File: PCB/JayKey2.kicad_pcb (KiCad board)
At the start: 4 copper layers, 1 part, among them U1 ATXMEGA128A1U-AU

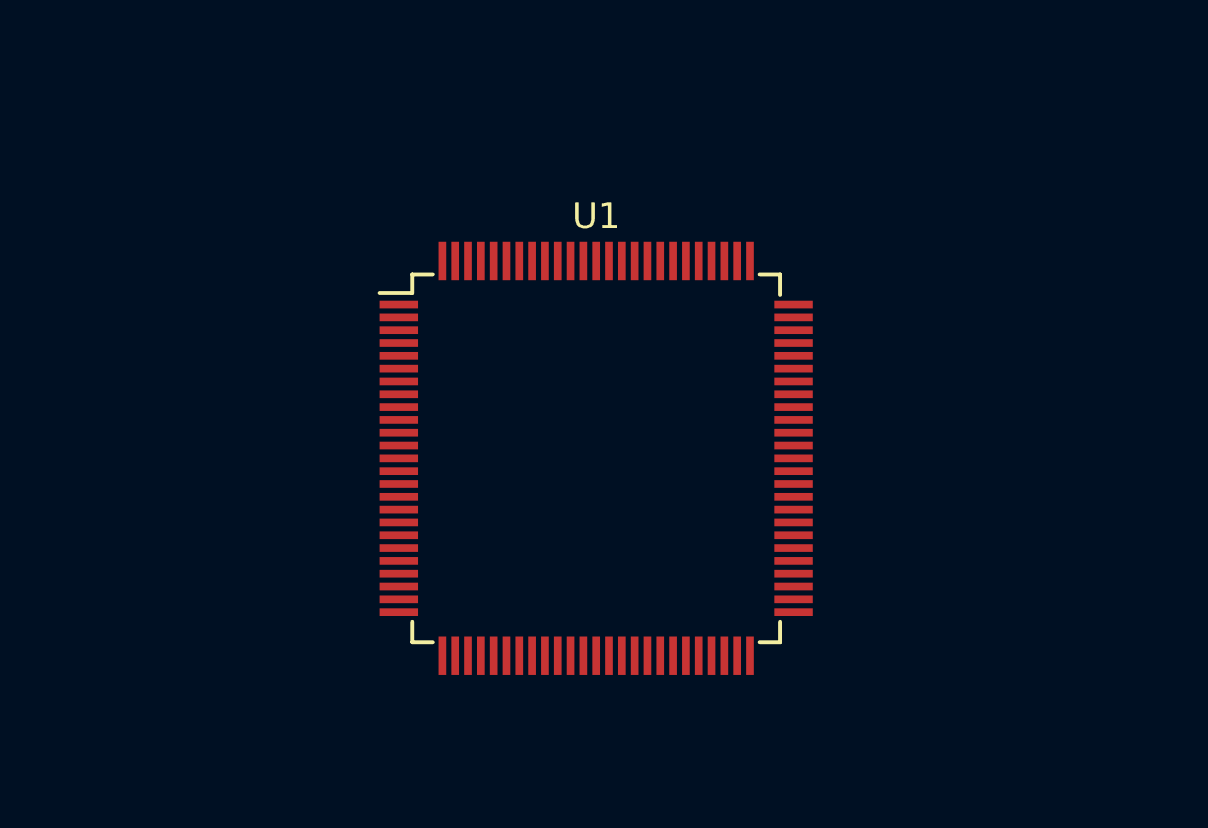
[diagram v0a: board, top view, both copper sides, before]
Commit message: 2018.03.29 Nightly
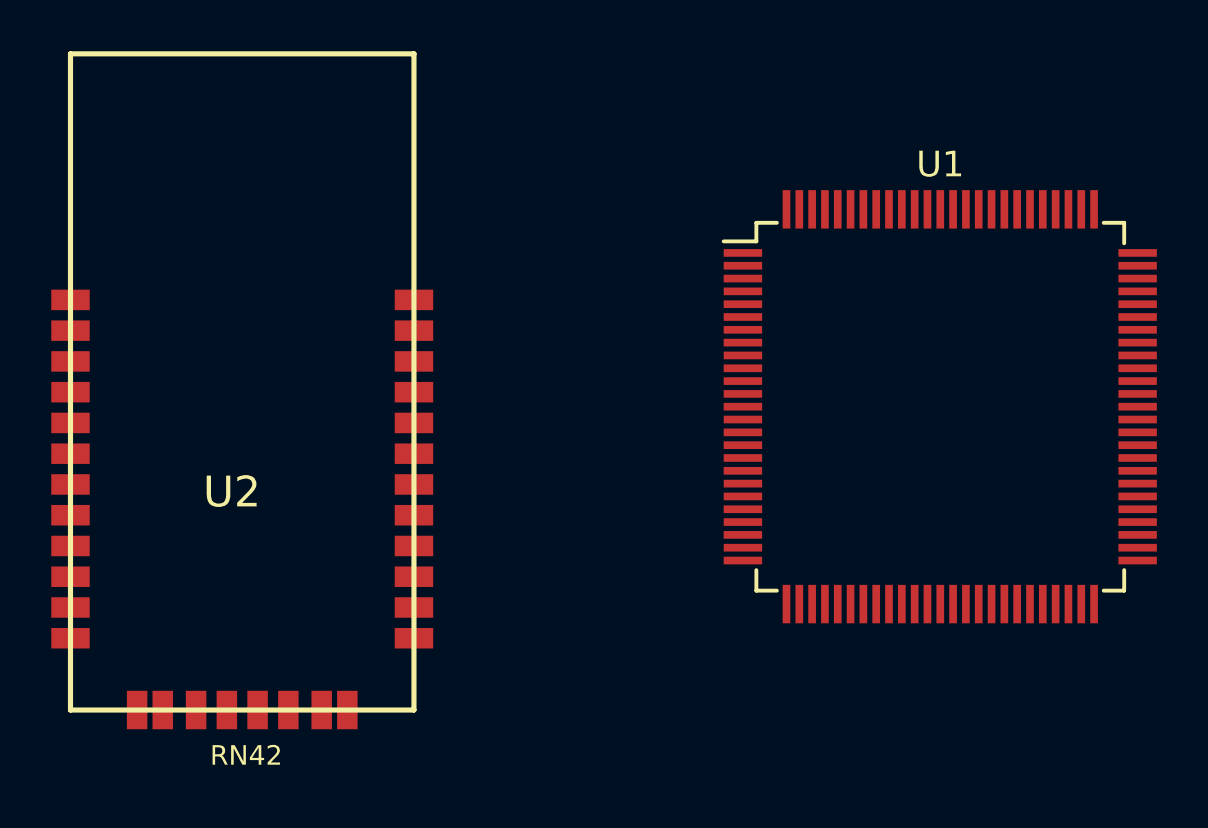
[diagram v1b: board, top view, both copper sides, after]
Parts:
- added U2: RN42, keyboard_parts:RN42, F.Cu at (128.0, 98.8)
- moved U1 13.6 mm to (161.9, 103.0)
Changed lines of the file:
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@@
     (links 0)
     (no_connects 0)
-    (area 139.576099 94.5786 157.426101 115.5286)
+    (area 127.042188 88.921874 170.850001 117.474975)
     (thickness 1.6)
     (drawings 0)
     (tracks 0)
     (zones 0)
-    (modules 1)
+    (modules 2)
     (nets 1)
   )
@@
   )
   (module Housings_QFP:TQFP-100_14x14mm_Pitch0.5mm (layer F.Cu)
-    (at 148.5011 105.0036)
+    (at 161.925 102.989063)
     (descr "100-Lead Plastic Thin Quad Flatpack (PF) - 14x14x1 mm Body 2.00 mm Footprint [TQFP] (see Microchip Packaging Specification 00000049BS.pdf)")
     (tags "QFP 0.5")
@@
     )
   )
+  (module keyboard_parts:RN42 (layer F.Cu)
+    (at 127.992188 98.821875)
+    (fp_text reference U2 (at 6.3 7.5) (layer F.SilkS)
+      (effects (font (size 1.2 1.2) (thickness 0.2)))
+    )
+    (fp_text value RN42 (at 6.858 17.78) (layer F.SilkS)
+      (effects (font (size 0.762 0.762) (thickness 0.127)))
+    )
+    (fp_line (start 13.4 16) (end 0 16) (layer F.SilkS) (width 0.2))
+    (fp_line (start 0 16) (end 0 -9.6) (layer F.SilkS) (width 0.2))
+    (fp_line (start 0 -9.6) (end 13.4 -9.6) (layer F.SilkS) (width 0.2))
+    (fp_line (start 13.4 -9.6) (end 13.4 16) (layer F.SilkS) (width 0.2))
+    (pad 11 smd rect (at 0 12) (size 1.5 0.8) (layers F.Cu F.Paste F.Mask))
+    (pad 12 smd rect (at 0 13.2) (size 1.5 0.8) (layers F.Cu F.Paste F.Mask))
+    (pad 10 smd rect (at 0 10.8) (size 1.5 0.8) (layers F.Cu F.Paste F.Mask))
+    (pad 9 smd rect (at 0 9.6) (size 1.5 0.8) (layers F.Cu F.Paste F.Mask))
+    (pad 5 smd rect (at 0 4.8) (size 1.5 0.8) (layers F.Cu F.Paste F.Mask))
+    (pad 6 smd rect (at 0 6) (size 1.5 0.8) (layers F.Cu F.Paste F.Mask))
+    (pad 8 smd rect (at 0 8.4) (size 1.5 0.8) (layers F.Cu F.Paste F.Mask))
+    (pad 7 smd rect (at 0 7.2) (size 1.5 0.8) (layers F.Cu F.Paste F.Mask))
+    (pad 3 smd rect (at 0 2.4) (size 1.5 0.8) (layers F.Cu F.Paste F.Mask))
+    (pad 4 smd rect (at 0 3.6) (size 1.5 0.8) (layers F.Cu F.Paste F.Mask))
+    (pad 2 smd rect (at 0 1.2) (size 1.5 0.8) (layers F.Cu F.Paste F.Mask))
+    (pad 1 smd rect (at 0 0) (size 1.5 0.8) (layers F.Cu F.Paste F.Mask))
+    (pad 13 smd rect (at 13.4 13.2) (size 1.5 0.8) (layers F.Cu F.Paste F.Mask))
+    (pad 14 smd rect (at 13.4 12) (size 1.5 0.8) (layers F.Cu F.Paste F.Mask))
+    (pad 15 smd rect (at 13.4 10.8) (size 1.5 0.8) (layers F.Cu F.Paste F.Mask))
+    (pad 16 smd rect (at 13.4 9.6) (size 1.5 0.8) (layers F.Cu F.Paste F.Mask))
+    (pad 17 smd rect (at 13.4 8.4) (size 1.5 0.8) (layers F.Cu F.Paste F.Mask))
+    (pad 18 smd rect (at 13.4 7.2) (size 1.5 0.8) (layers F.Cu F.Paste F.Mask))
+    (pad 19 smd rect (at 13.4 6) (size 1.5 0.8) (layers F.Cu F.Paste F.Mask))
+    (pad 20 smd rect (at 13.4 4.8) (size 1.5 0.8) (layers F.Cu F.Paste F.Mask))
+    (pad 21 smd rect (at 13.4 3.6) (size 1.5 0.8) (layers F.Cu F.Paste F.Mask))
+    (pad 22 smd rect (at 13.4 2.4) (size 1.5 0.8) (layers F.Cu F.Paste F.Mask))
+    (pad 23 smd rect (at 13.4 1.2) (size 1.5 0.8) (layers F.Cu F.Paste F.Mask))
+    (pad 24 smd rect (at 13.4 0) (size 1.5 0.8) (layers F.Cu F.Paste F.Mask))
+    (pad 35 smd rect (at 2.6 16) (size 0.8 1.5) (layers F.Cu F.Paste F.Mask)
+      (clearance 0.1778))
+    (pad 29 smd rect (at 3.6 16) (size 0.8 1.5) (layers F.Cu F.Paste F.Mask)
+      (clearance 0.1778))
+    (pad 34 smd rect (at 4.9 16) (size 0.8 1.5) (layers F.Cu F.Paste F.Mask))
+    (pad 33 smd rect (at 6.1 16) (size 0.8 1.5) (layers F.Cu F.Paste F.Mask))
+    (pad 32 smd rect (at 7.3 16) (size 0.8 1.5) (layers F.Cu F.Paste F.Mask))
+    (pad 31 smd rect (at 8.5 16) (size 0.8 1.5) (layers F.Cu F.Paste F.Mask))
+    (pad 28 smd rect (at 9.8 16) (size 0.8 1.5) (layers F.Cu F.Paste F.Mask)
+      (clearance 0.1778))
+    (pad 30 smd rect (at 10.8 16) (size 0.8 1.5) (layers F.Cu F.Paste F.Mask)
+      (clearance 0.1778))
+  )
 )
